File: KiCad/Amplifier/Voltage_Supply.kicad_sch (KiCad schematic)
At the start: 10 parts, among them J3 Vp_8V, J4 Vn_-5V

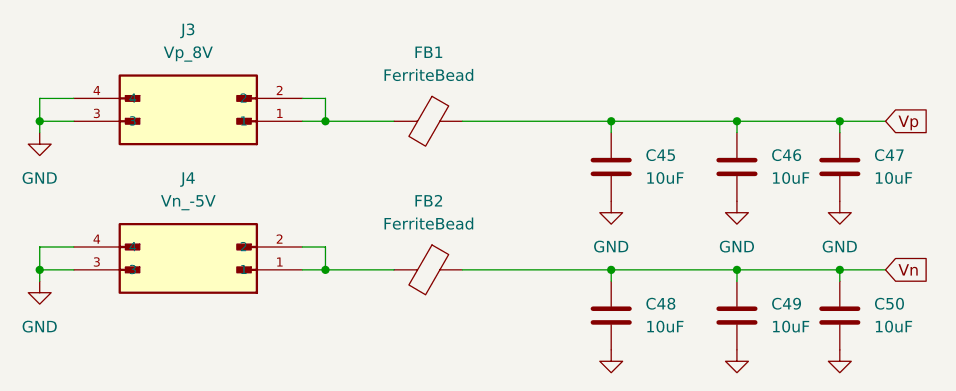
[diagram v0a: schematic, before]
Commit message: Update PCB
update PCB
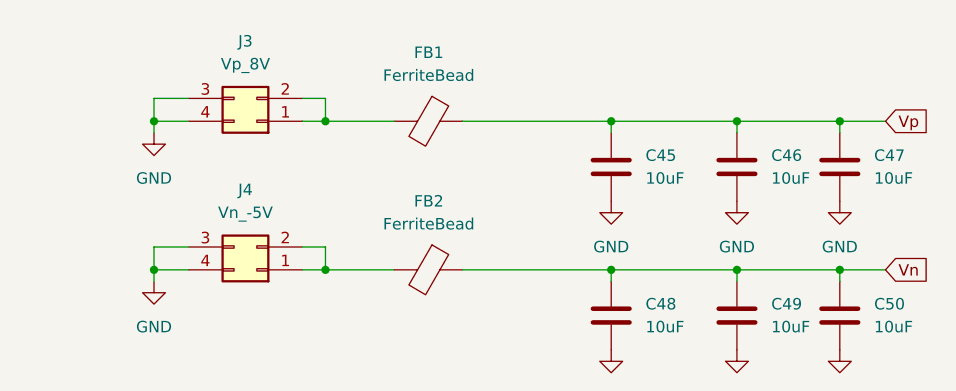
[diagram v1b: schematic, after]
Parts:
- removed J3: Vp_8V, Library:MOLEX_26013115, symbol New_Library_0:Molex_26013115
- removed J4: Vn_-5V, Library:MOLEX_26013115, symbol New_Library_0:Molex_26013115
- added J3: Vp_8V, Library:MOLEX_26013115, symbol Connector_Generic:Conn_02x02_Counter_Clockwise
- added J4: Vn_-5V, Library:MOLEX_26013115, symbol Connector_Generic:Conn_02x02_Counter_Clockwise
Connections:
- net GND: now also J3.3 (Pin_3), J3.4 (Pin_4), J4.3 (Pin_3), J4.4 (Pin_4)
- net at FB1.2: now also J3.1 (Pin_1), J3.2 (Pin_2)
- net at FB2.2: now also J4.1 (Pin_1), J4.2 (Pin_2)
